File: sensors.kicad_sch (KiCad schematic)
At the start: 5 parts, among them U1 LIS3MDL, U2 MAX-M10S

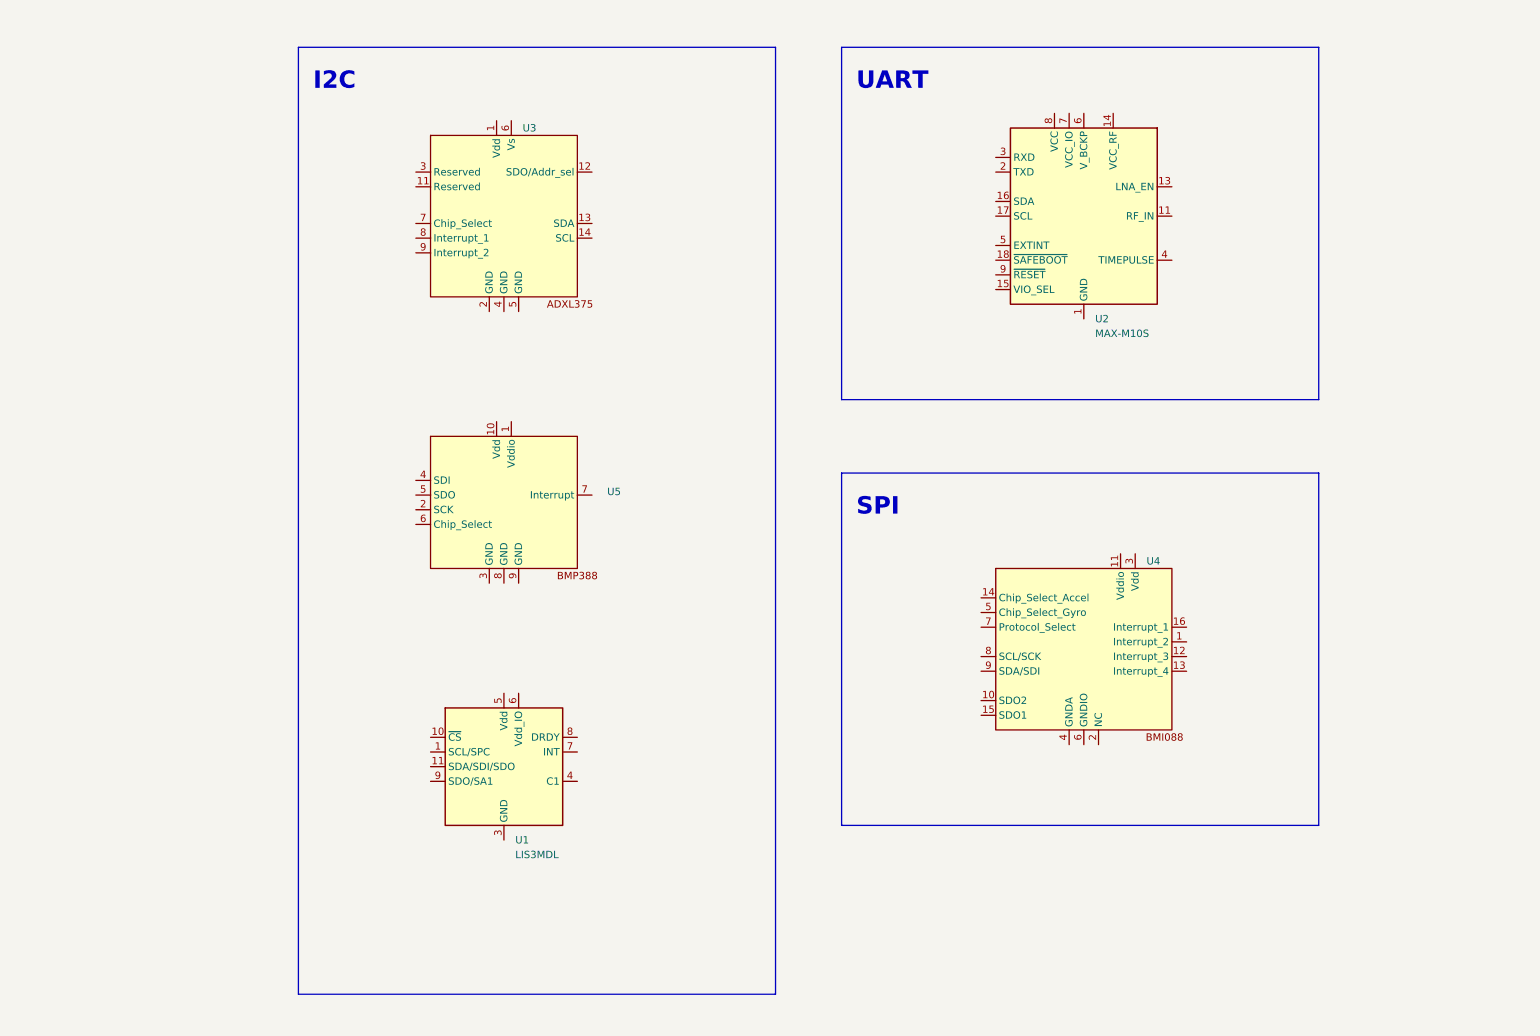
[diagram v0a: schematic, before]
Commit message: Finished Updating Sensor Schematics
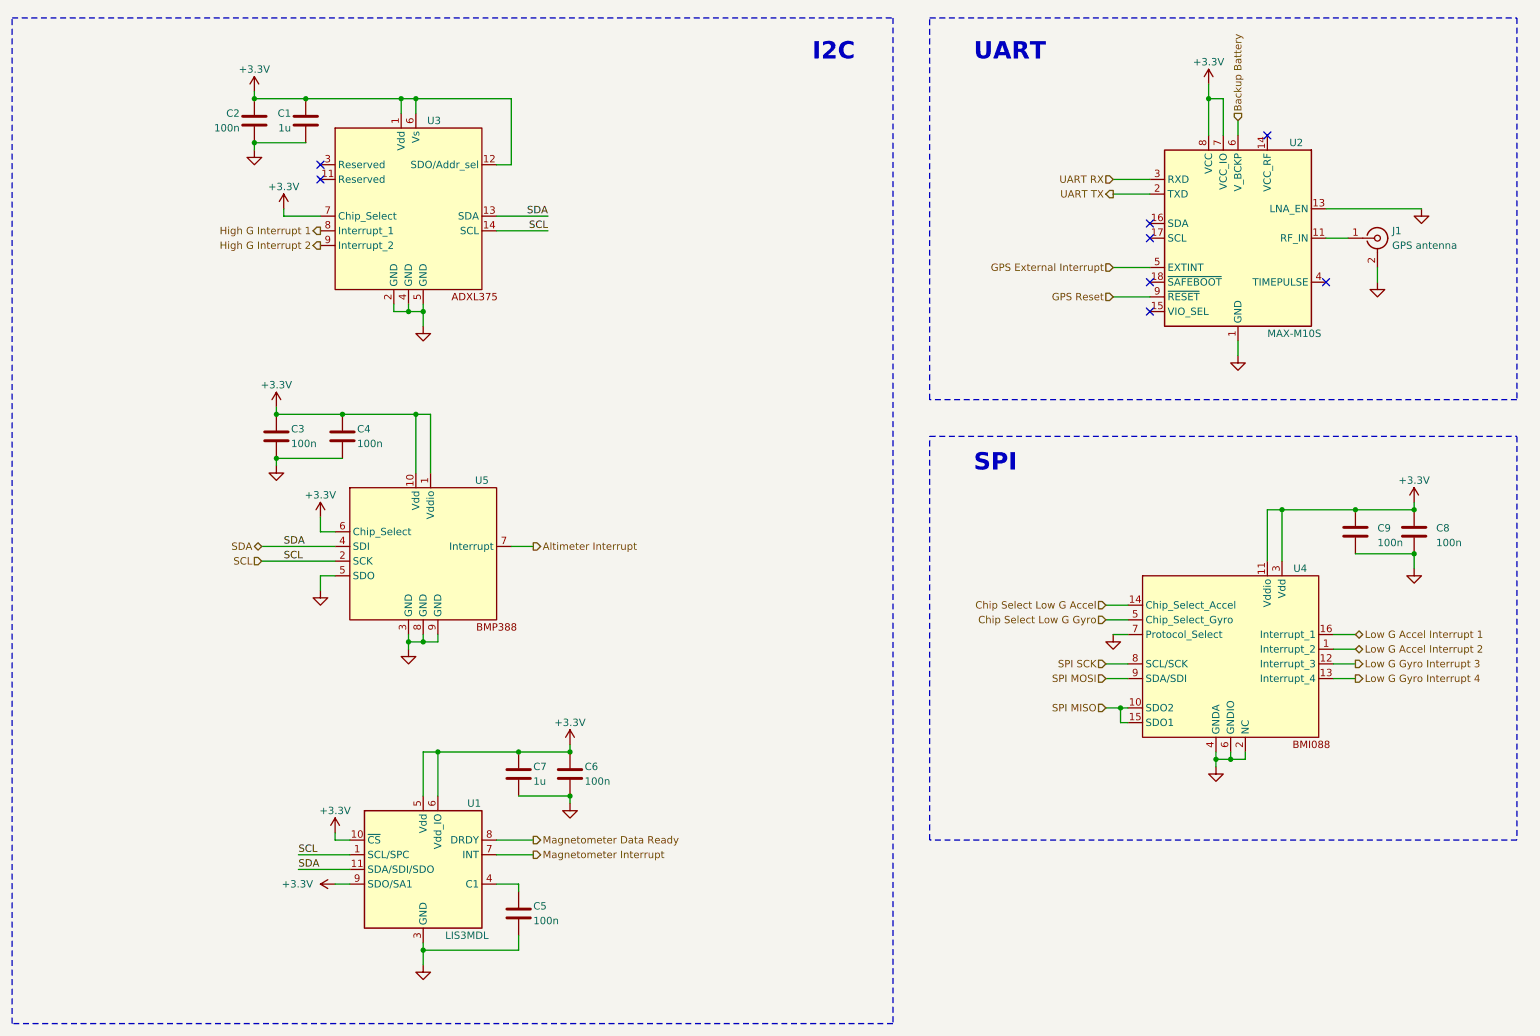
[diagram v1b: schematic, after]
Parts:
- added C1, C7: 1u, symbol Device:C
- added C2, C3, C4, C5, C6, C8, C9: 100n, symbol Device:C
- added J1: GPS antenna, symbol Connector:Conn_Coaxial
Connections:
- net +3.3V: now reaches U3.1 (Vdd)
- net +3.3V: now also U1.10 (~{CS}), U1.5 (Vdd), U1.6 (Vdd_IO), U1.9 (SDO/SA1), U2.7 (VCC_IO), U2.8 (VCC), U3.12 (SDO/Addr_sel), U3.6 (Vs), U3.7 (Chip_Select), U4.11 (Vddio), U4.3 (Vdd), U5.1 (Vddio), U5.10 (Vdd), U5.6 (Chip_Select), C1.1, C2.1, C3.1, C4.1, C6.1, C7.1, C8.1, C9.1
- net SDA: now reaches U3.13 (SDA)
- net SDA: now also U1.11 (SDA/SDI/SDO), U5.4 (SDI)
- net SCL: now reaches U3.14 (SCL)
- net SCL: now also U1.1 (SCL/SPC), U5.2 (SCK)
- net GND: now reaches U3.2 (GND)
- net GND: now also U1.12 (GND), U1.2 (GND), U1.3 (GND), U2.1 (GND), U2.10 (GND), U2.12 (GND), U2.13 (LNA_EN), U3.4 (GND), U3.5 (GND), U4.2 (NC), U4.4 (GNDA), U4.6 (GNDIO), U4.7 (Protocol_Select), U5.3 (GND), U5.5 (SDO), U5.8 (GND), U5.9 (GND), C1.2, C2.2, C3.2, C4.2, C5.2, C6.2, C7.2, C8.2, C9.2, J1.2 (Ext)
- net High G Interrupt 1: now reaches U3.8 (Interrupt_1)
- net High G Interrupt 2: now reaches U3.9 (Interrupt_2)
- net at U1.4 (C1): now also C5.1
- net Magnetometer Interrupt: now reaches U1.7 (INT)
- net Magnetometer Data Ready: now reaches U1.8 (DRDY)
- net at U2.11 (RF_IN): now also J1.1 (In)
- net UART TX: now reaches U2.2 (TXD)
- net UART RX: now reaches U2.3 (RXD)
- net GPS External Interrupt: now reaches U2.5 (EXTINT)
- net Backup Battery: now reaches U2.6 (V_BCKP)
- net GPS Reset: now reaches U2.9 (~{RESET})
- net Low G Accel Interrupt 2: now reaches U4.1 (Interrupt_2)
- net SPI MISO: now reaches U4.10 (SDO2)
- net SPI MISO: now also U4.15 (SDO1)
- net Low G Gyro Interrupt 3: now reaches U4.12 (Interrupt_3)
- net Low G Gyro Interrupt 4: now reaches U4.13 (Interrupt_4)
- net Chip Select Low G Accel: now reaches U4.14 (Chip_Select_Accel)
- net Low G Accel Interrupt 1: now reaches U4.16 (Interrupt_1)
- net Chip Select Low G Gyro: now reaches U4.5 (Chip_Select_Gyro)
- net SPI SCK: now reaches U4.8 (SCL/SCK)
- net SPI MOSI: now reaches U4.9 (SDA/SDI)
- net Altimeter Interrupt: now reaches U5.7 (Interrupt)
- no-connect marks 0 -> 8
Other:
- moved on the sheet: U1, U2, U3, U4
